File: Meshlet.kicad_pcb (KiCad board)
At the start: 2 copper layers, 60.2 x 39 mm, 114 parts, among them J1 Ext. Notif. Header, J10 STEMMA QT I2C, J11 GPIO Exp., J12 I2C PINHEADER, J13 Ext. Power Header, J2 USB_C_Receptacle_USB2.0_16P, J3 Ext. Power Header, J4 Batt. Header (JST-PH 2.0), J5 SWD, J6 Batt. Header (Picoblade 1.25), J7 GPS Header, J8 User Btn Header, J9 Power Switch, Q1 AO3400A, SW1 BOOTSEL, SW3 RST, U1 W25Q32JVZP, U10 XC6206PxxxMR, U11 XC6206PxxxMR, U2 XC6206PxxxMR, U3 RP2350_60QFN, U4 INA3221, U5 BME280, U6 Wio-SX1262, U7 USBLC6-2SC6, U8 BQ24074RGT, Y1 12.000MHz

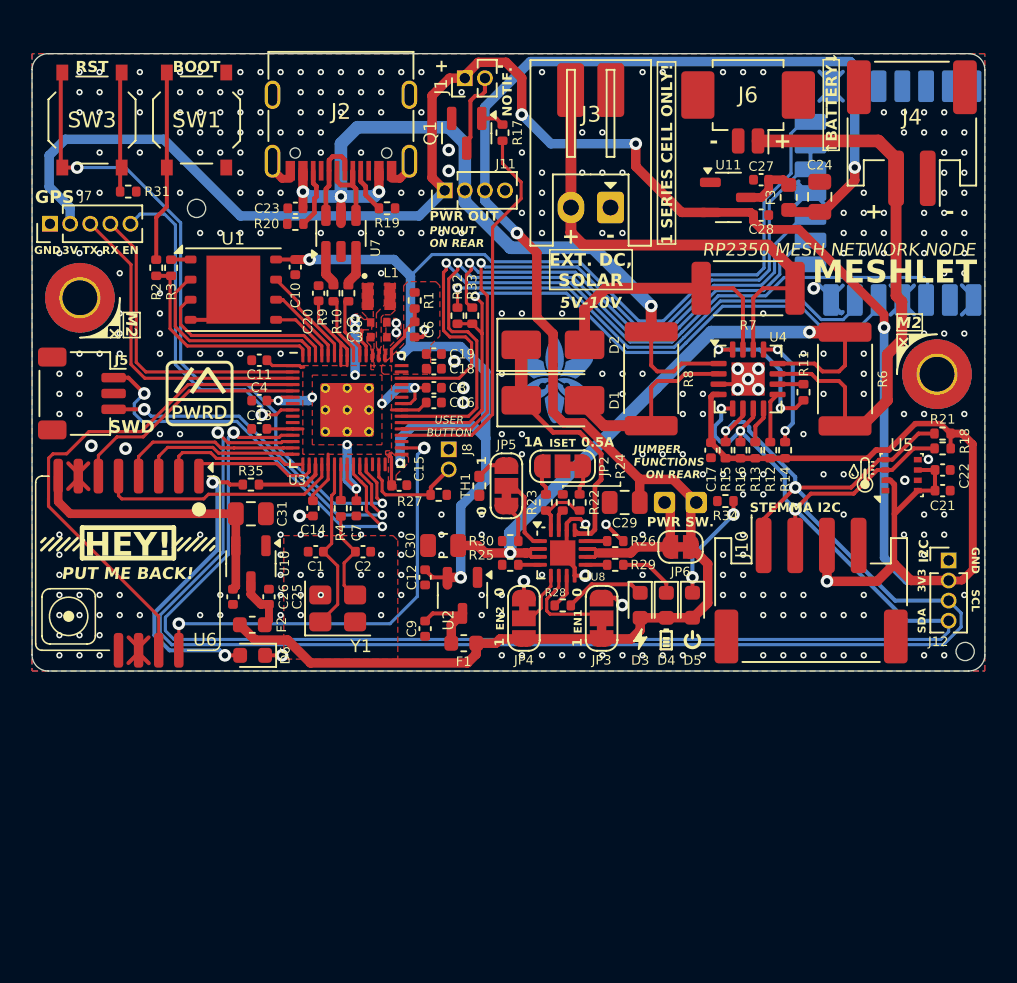
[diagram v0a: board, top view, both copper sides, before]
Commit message: Redesign!
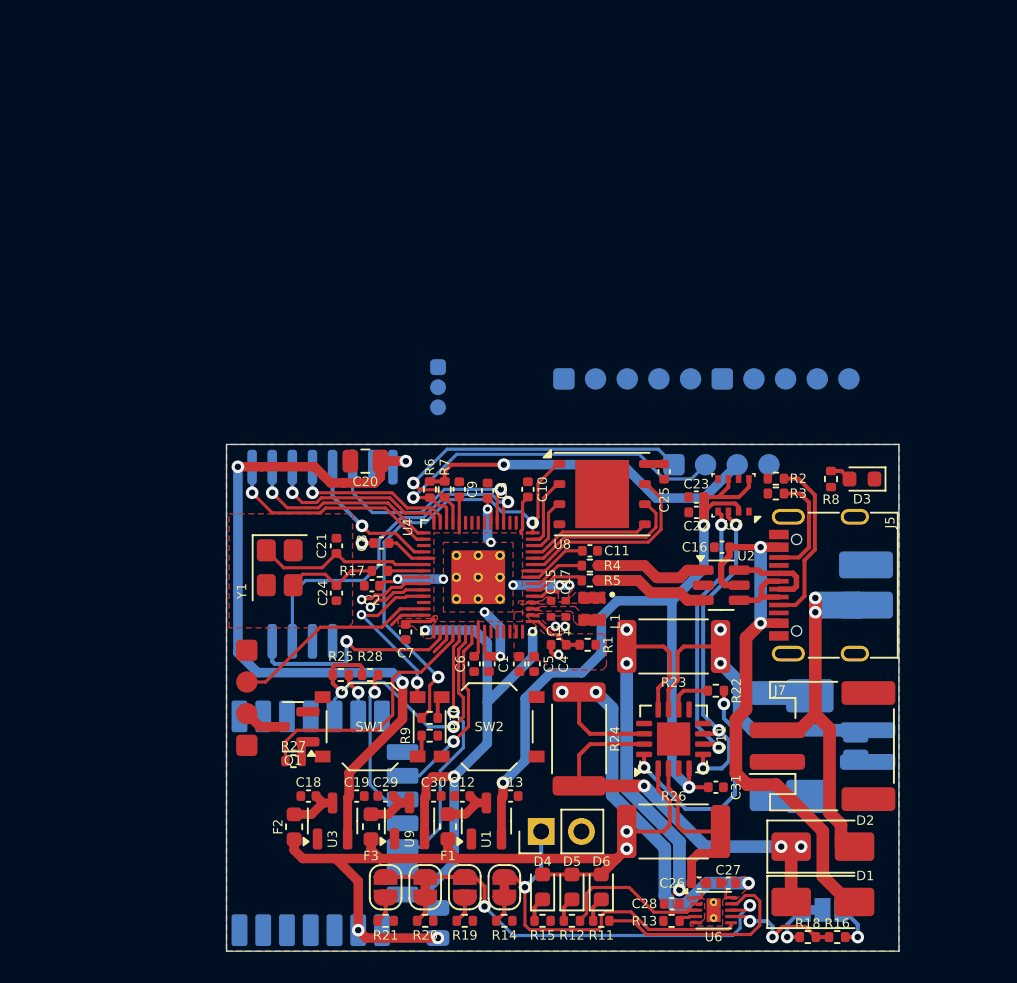
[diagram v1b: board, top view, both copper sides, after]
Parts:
- removed G***: LOGO, Graphics:HalftoneOverlay
- removed J10: STEMMA QT I2C, Connector_JST:JST_PH_S4B-PH-SM4-TB_1x04-1MP_P2.00mm_Horizontal
- removed J8: User Btn Header, Connector_PinHeader_1.27mm:PinHeader_1x02_P1.27mm_Vertical
- removed JP6: PwrSw Bypass, Jumper:SolderJumper-2_P1.3mm_Bridged_RoundedPad1.0x1.5mm
- removed R29, R30, R33, R34, R35: 10k, Resistor_SMD:R_0402_1005Metric
- removed R31: 1k, Resistor_SMD:R_0402_1005Metric
- removed R32: 470R, Resistor_SMD:R_0402_1005Metric
- removed REF** (x2): MountingHole_2.2mm_M2_Pad_TopBottom, MountingHole:MountingHole_2.2mm_M2_Pad_TopBottom
- removed REF** (x2): ToolingHole_1.152mm, MountingHole:ToolingHole_1.152mm
- removed SW3: RST, Button_Switch_SMD:SW_Push_1P1T_XKB_TS-1187A
- removed TH1: Thermistor_NTC, Resistor_SMD:R_0402_1005Metric_Pad0.72x0.64mm_HandSolder
- added C32: 47uF, Capacitor_SMD:C_0805_2012Metric, B.Cu at (135.9, 109.1)
- added J14: Ext. Notif. Header, Connector_PinHeader_2.00mm:PinHeader_1x02_P2.00mm_Vertical, F.Cu at (123.8, 97.9)
- added JP1: TS, Jumper:SolderJumper-2_P1.3mm_Bridged_RoundedPad1.0x1.5mm, F.Cu at (140.1, 106.8)
- added R5: 27R, Resistor_SMD:R_0402_1005Metric, F.Cu at (145.5, 87.5)
- added SW2: BOOTSEL, Button_Switch_SMD:SW_Push_1P1T_XKB_TS-1187A, F.Cu at (139.1, 96.7)
- C1: value 15pF -> 100nF
- C13, C18, C19: value 100nF -> 1uF
- C14: value 100nF -> 4.7uF
- C15, C17: value 100nF -> 4.7uF; footprint Capacitor_SMD:C_0402_1005Metric -> RP2350 Components:C_0402_1005Metric_small_pads
- C2: value 15pF -> 4.7uF
- C20: value 100nF -> 47uF; footprint Capacitor_SMD:C_0402_1005Metric -> Capacitor_SMD:C_0805_2012Metric
- C21: value 100nF -> 15pF
- C24: value 47uF -> 15pF; footprint Capacitor_SMD:C_0805_2012Metric -> Capacitor_SMD:C_0402_1005Metric
- C25, C9: value 1uF -> 100nF
- C26, C27, C28: value 1uF -> 22uF
- C29, C30: value 47uF -> 1uF; footprint Capacitor_SMD:C_0805_2012Metric -> Capacitor_SMD:C_0402_1005Metric
- C3, C5: value 4.7uF -> 100nF; footprint RP2350 Components:C_0402_1005Metric_small_pads -> Capacitor_SMD:C_0402_1005Metric
- C31: value 47uF -> 100nF; footprint Capacitor_SMD:C_0805_2012Metric -> Capacitor_SMD:C_0402_1005Metric
- C6, C7: value 4.7uF -> 100nF
- D3: value PG -> HB
- D4: value CHG -> PV
- D5: value PWR -> CHG
- D6: value HB -> FLT
- J1: value Ext. Notif. Header -> SWD; footprint Connector_PinHeader_1.27mm:PinHeader_1x02_P1.27mm_Vertical -> Connector_PinHeader_1.27mm:PinHeader_1x03_P1.27mm_Vertical; moved to B.Cu
- J11: footprint Connector_PinHeader_1.27mm:PinHeader_1x04_P1.27mm_Vertical -> Connector_PinHeader_2.00mm:PinHeader_1x05_P2.00mm_Vertical; moved to B.Cu
- J12: value I2C PINHEADER -> GPS Header; footprint Connector_PinHeader_1.27mm:PinHeader_1x04_P1.27mm_Vertical -> Connector_PinHeader_2.00mm:PinHeader_1x05_P2.00mm_Vertical; moved to B.Cu
- J13: value Ext. Power Header -> Thermistor Pins
- J2: value USB_C_Receptacle_USB2.0_16P -> User Btn Header; footprint Connector_USB:USB_C_Receptacle_G-Switch_GT-USB-7010ASV -> Connector_PinHeader_2.00mm:PinHeader_1x02_P2.00mm_Vertical
- J3: value Ext. Power Header -> Batt. Header (Picoblade 1.25); footprint Connector_JST:JST_XH_S2B-XH-A_1x02_P2.50mm_Horizontal -> Connector_Molex:Molex_PicoBlade_53261-0271_1x02-1MP_P1.25mm_Horizontal; moved to B.Cu
- J4: moved to B.Cu
- J5: value SWD -> USB_C_Receptacle_USB2.0_16P; footprint Connector_JST:JST_SH_SM03B-SRSS-TB_1x03-1MP_P1.00mm_Horizontal -> Connector_USB:USB_C_Receptacle_G-Switch_GT-USB-7010ASV
- J6: value Batt. Header (Picoblade 1.25) -> STEMMA QT I2C; footprint Connector_Molex:Molex_PicoBlade_53261-0271_1x02-1MP_P1.25mm_Horizontal -> Connector_PinHeader_2.00mm:PinHeader_1x04_P2.00mm_Vertical; moved to B.Cu
- J7: value GPS Header -> Ext. Power Header; footprint Connector_PinHeader_1.27mm:PinHeader_1x05_P1.27mm_Vertical -> Connector_JST:JST_PH_S2B-PH-SM4-TB_1x02-1MP_P2.00mm_Horizontal
- J9: value Power Switch -> Ext. Power Header; footprint Connector_PinHeader_2.00mm:PinHeader_1x02_P2.00mm_Vertical -> Connector_PinHeader_2.54mm:PinHeader_1x02_P2.54mm_Vertical; moved to B.Cu
- JP2: value ISET -> Chemistry Select; moved to B.Cu
- JP3: value EN1 -> SolderJumper_2_Open; footprint Jumper:SolderJumper-3_P1.3mm_Bridged12_RoundedPad1.0x1.5mm -> Jumper:SolderJumper-2_P1.3mm_Open_RoundedPad1.0x1.5mm
- JP4: value EN2 -> SolderJumper_2_Bridged; footprint Jumper:SolderJumper-3_P1.3mm_Bridged12_RoundedPad1.0x1.5mm -> Jumper:SolderJumper-2_P1.3mm_Bridged_RoundedPad1.0x1.5mm
- JP5: value Jumper_3_Bridged12 -> SolderJumper_2_Open; footprint Jumper:SolderJumper-3_P1.3mm_Bridged12_RoundedPad1.0x1.5mm -> Jumper:SolderJumper-2_P1.3mm_Open_RoundedPad1.0x1.5mm
- R10, R9: value 27R -> 1k
- R16: value 10k -> 13k
- R17: value 10k -> 1k
- R18: value 4.7k -> 5.1k
- R19: value 5.1k -> 300
- R2: value 1k -> 5.1k
- R20: value 5.1k -> 600
- R21: value 4.7k -> 1.2k
- R23, R26: value 1k -> PA2512FKF7W0R01E; footprint Resistor_SMD:R_0402_1005Metric -> Resistor_SMD:R_2512_6332Metric
- R24: value 10k -> PA2512FKF7W0R01E; footprint Resistor_SMD:R_0402_1005Metric -> Resistor_SMD:R_2512_6332Metric
- R25: value 10k -> 470R
- R27: value 1k -> 10k
- R3: value 0 -> 5.1k
- R4: value 1k -> 27R
- R6, R7, R8: value PA2512FKF7W0R01E -> 10k; footprint Resistor_SMD:R_2512_6332Metric -> Resistor_SMD:R_0402_1005Metric
- SW1: value BOOTSEL -> RST
- U1: value W25Q32JVZP -> XC6206PxxxMR; footprint Package_SON:WSON-8-1EP_6x5mm_P1.27mm_EP3.4x4.3mm -> Package_TO_SOT_SMD:SOT-23-3
- U10: value XC6206PxxxMR -> ~; footprint Package_TO_SOT_SMD:SOT-23-3 -> RM2:Radio Module 2; moved to B.Cu
- U11: value XC6206PxxxMR -> INA3221; footprint Package_TO_SOT_SMD:SOT-23-3 -> Package_DFN_QFN:Texas_RGV0016A_VQFN-16-1EP_4x4mm_P0.65mm_EP2.1x2.1mm
- U2: value XC6206PxxxMR -> USBLC6-2SC6; footprint Package_TO_SOT_SMD:SOT-23-3 -> Package_TO_SOT_SMD:SOT-23-6
- U3: value RP2350_60QFN -> XC6206PxxxMR; footprint RP2350_60QFN_minimal:RP2350-QFN-60-1EP_7x7_P0.4mm_EP3.4x3.4mm_ThermalVias -> Package_TO_SOT_SMD:SOT-23-3
- U4: value INA3221 -> RP2350_60QFN; footprint Package_DFN_QFN:Texas_RGV0016A_VQFN-16-1EP_4x4mm_P0.65mm_EP2.1x2.1mm -> RP2350_60QFN_minimal:RP2350-QFN-60-1EP_7x7_P0.4mm_EP3.4x3.4mm_ThermalVias
- U5: value BME280 -> Wio-SX1262; footprint Package_LGA:Bosch_LGA-8_2.5x2.5mm_P0.65mm_ClockwisePinNumbering -> Wio-SX1262:Wio-SX1262; moved to B.Cu
- U6: value Wio-SX1262 -> BQ25185; footprint Wio-SX1262:Wio-SX1262 -> Package_DFN_QFN:Texas_DLH0010A_WSON-10-1EP_2.2x2mm_P0.4mm_EP0.9x1.5mm_ThermalVias
- U7: value USBLC6-2SC6 -> BME280; footprint Package_TO_SOT_SMD:SOT-23-6 -> Package_LGA:Bosch_LGA-8_2.5x2.5mm_P0.65mm_ClockwisePinNumbering
- U8: value BQ24074RGT -> W25Q32JVZP; footprint Package_DFN_QFN:VQFN-16-1EP_3x3mm_P0.5mm_EP1.6x1.6mm -> Package_SON:WSON-8-1EP_6x5mm_P1.27mm_EP3.4x4.3mm
- U9: value ~ -> XC6206PxxxMR; footprint RM2:Radio Module 2 -> Package_TO_SOT_SMD:SOT-23-3; moved to F.Cu
- moved J7 58.9 mm to (160.2, 97.9)
- moved U9 57.4 mm to (134.1, 102.6)
- moved J5 49.3 mm to (161.2, 87.7), turned to 90 degrees
- moved F3 47.7 mm to (131.7, 103.0)
- moved J13 47.0 mm to (142.4, 103.3), turned to 90 degrees
- moved R21 46.7 mm to (132.6, 108.9), turned to 180 degrees
- moved R19 45.3 mm to (137.6, 108.9), turned to 180 degrees
- moved R20 44.8 mm to (135.1, 108.9), turned to 180 degrees
- moved C27 44.5 mm to (154.2, 106.6)
- moved C28 43.9 mm to (150.7, 107.9), turned to 180 degrees
- moved U6 43.0 mm to (153.3, 108.3), turned to 0 degrees
- moved U5 42.3 mm to (122.8, 80.3), turned to 0 degrees
- moved R2 41.3 mm to (157.2, 81.0), turned to 180 degrees
- moved R3 40.8 mm to (157.2, 82.0), turned to 0 degrees
- moved SW1 39.9 mm to (131.6, 96.7), turned to 0 degrees
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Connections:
- C1 pad 1: GND -> +1V1
- C1 pad 2: XIN -> GND
- C12 pad 1: /Pi +3V3 -> Net-(U1-VI)
- C13 pad 1: /Pi +3V3 -> +3V3
- C14 pad 1: /Pi +3V3 -> Net-(U4-VREG_AVDD)
- C16 pad 1: /Pi +3V3 -> USB_RAW
- C17 pad 1: GND -> +1V1
- C17 pad 2: +3V3 -> GND
- C18 pad 1: /Pi +3V3 -> Net-(U3-VI)
- C19 pad 1: /Pi +3V3 -> /LoRa +3V3
- C2 pad 1: GND -> +1V1
- C2 pad 2: Net-(C2-Pad2) -> GND
- C20 pad 1: /Pi +3V3 -> GND
- C20 pad 2: GND -> /LoRa +3V3
- C21 pad 1: +3V3 -> GND
- C21 pad 2: GND -> XIN
- C23 pad 1: INA_IN3- -> +3V3
- C24 pad 2: BMS_OUT -> Net-(C24-Pad2)
- C25 pad 1: Net-(U10-VI) -> /Pi +3V3
- C26 pad 1: /LoRa +3V3 -> BMS_INA
- C27 pad 1: Net-(U11-VI) -> VBUS_OUT
- C28 pad 1: +3V3 -> BATT
- C29 pad 1: BMS_OUT -> Net-(U9-VI)
- C3 pad 1: /Pi +3V3 -> +1V1
- C30 pad 1: INA_IN1+ -> /Pi +3V3
- C31 pad 2: /LoRa +3V3 -> +3V3
- C4 pad 1: +1V1 -> /Pi +3V3
- C5 pad 1: +1V1 -> /Pi +3V3
- C6 pad 1: Net-(U3-VREG_AVDD) -> /Pi +3V3
- C7 pad 1: +1V1 -> /Pi +3V3
- C8 pad 1: +1V1 -> /Pi +3V3
- C9 pad 1: Net-(U2-VI) -> /Pi +3V3
- D1 pad 1: VBUS -> VBUS_INA
- D1 pad 2: INA_IN3+ -> USB_RAW
- D2 pad 1: VBUS -> VBUS_INA
- D2 pad 2: INA_IN2+ -> Net-(D2-A)
- D3 pad 1: Net-(D3-K) -> GND
- D3 pad 2: BMS_OUT -> Net-(D3-A)
- D6 pad 1: GND -> Net-(D6-K)
- D6 pad 2: Net-(D6-A) -> BMS_OUT
- F1 pad 2: Net-(U2-VI) -> Net-(U1-VI)
- F2 pad 2: Net-(U10-VI) -> Net-(U3-VI)
- F3 pad 2: Net-(U11-VI) -> Net-(U9-VI)
- J1 pad 1: +3V3 -> SWCLK
- J1 pad 2: Net-(J1-Pin_2) -> GND
- J11 pad 1: +3V3 -> GP4
- J11 pad 2: INA_IN3- -> GP16
- J11 pad 3: BMS_OUT -> GP18
- J11 pad 4: GND -> GP19
- J12 pad 3: I2C_SCL -> GPS_TX
- J12 pad 4: I2C_SDA -> GPS_RX
- J13 pad 1: GND -> THERM
- J13 pad 2: INA_IN2- -> GND
- J3 pad 2: INA_IN2- -> BATT_INA
- J4 pad 2: INA_IN1- -> BATT_INA
- J6 pad 1: INA_IN1- -> I2C_SDA
- J6 pad 2: GND -> I2C_SCL
- J7 pad 2: +3V3 -> Net-(D2-A)
- J9 pad 1: Net-(J9-Pin_1) -> GND
- J9 pad 2: BMS_OUT -> Net-(D2-A)
- JP3 pad 1: BMS_OUT -> Net-(JP3-A)
- JP3 pad 2: BMS_EN1 -> ISET
- JP4 pad 1: GND -> Net-(JP4-A)
- JP4 pad 2: BMS_EN2 -> ISET
- JP5 pad 2: Net-(JP5-C) -> ISET
- L1 pad 2: Net-(U3-VREG_LX) -> Net-(U4-VREG_LX)
- Q1 pad 3: Net-(J1-Pin_2) -> Net-(J14-Pin_2)
- R1 pad 2: Net-(U3-VREG_AVDD) -> Net-(U4-VREG_AVDD)
- R10 pad 1: USB_DN -> Net-(R10-Pad1)
- R10 pad 2: Net-(U3-USB_DM) -> QSPI_SS
- R11 pad 1: INA_VPU -> Net-(U6-STAT1)
- R11 pad 2: INA_PV -> Net-(D6-K)
- R12 pad 1: +3V3 -> Net-(U6-STAT2)
- R12 pad 2: INA_CRIT -> Net-(D5-K)
- R13 pad 1: +3V3 -> GND
- R13 pad 2: INA_WARN -> Net-(U6-CE)
- R14 pad 1: +3V3 -> Net-(JP1-B)
- R14 pad 2: INA_TC -> GND
- R15 pad 1: +3V3 -> Net-(D4-K)
- R15 pad 2: I2C_SCL -> GND
- R16 pad 1: +3V3 -> VSET
- R16 pad 2: I2C_SDA -> Net-(JP2-B)
- R17 pad 1: NOTIFY -> Net-(C24-Pad2)
- R17 pad 2: Net-(Q1-G) -> XOUT
- R18 pad 1: I2C_SDA -> Net-(JP2-A)
- R18 pad 2: +3V3 -> VSET
- R19 pad 1: Net-(J2-CC1) -> GND
- R19 pad 2: GND -> Net-(JP3-A)
- R2 pad 1: Net-(R2-Pad1) -> Net-(J5-CC1)
- R2 pad 2: QSPI_SS -> GND
- R20 pad 2: Net-(J2-CC2) -> Net-(JP4-A)
- R21 pad 1: I2C_SCL -> GND
- R21 pad 2: +3V3 -> Net-(JP5-A)
- R22 pad 1: Net-(U8-ISET) -> INA_VPU
- R22 pad 2: Net-(JP2-A) -> INA_PV
- R23 pad 1: Net-(U8-ISET) -> BATT
- R23 pad 2: Net-(JP2-B) -> BATT_INA
- R24 pad 1: GND -> VBUS_INA
- R24 pad 2: Net-(U8-ITERM) -> VBUS_OUT
- R25 pad 1: Net-(U8-~{CE}) -> GP24
- R25 pad 2: GND -> Net-(U10-DO)
- R26 pad 1: GND -> BMS_INA
- R26 pad 2: Net-(U8-ILIM) -> BMS_OUT
- R27 pad 1: USER_BTN -> NOTIFY
- R27 pad 2: GND -> Net-(Q1-G)
- R28 pad 1: Net-(U8-~{PGOOD}) -> GP24
- R28 pad 2: Net-(D3-K) -> Net-(U10-IRQ)
- R3 pad 1: Net-(U1-~{CS}) -> GND
- R3 pad 2: QSPI_SS -> Net-(J5-CC2)
- R4 pad 1: Net-(C2-Pad2) -> USB_DP
- R4 pad 2: XOUT -> Net-(U4-USB_DP)
- R6 pad 1: INA_IN1+ -> +3V3
- R6 pad 2: INA_IN1- -> I2C_SCL
- R7 pad 1: INA_IN2+ -> +3V3
- R7 pad 2: INA_IN2- -> I2C_SDA
- R8 pad 1: INA_IN3+ -> Net-(D3-A)
- R8 pad 2: INA_IN3- -> Net-(U4-GPIO14)
- R9 pad 1: USB_DP -> Net-(R9-Pad1)
- R9 pad 2: Net-(U3-USB_DP) -> GND
- SW1 pad 1: Net-(R2-Pad1) -> Net-(U4-RUN)
- SW1 pad 2: GND -> Net-(R9-Pad1)
- U1 pad 1: Net-(U1-~{CS}) -> GND
- U1 pad 2: QSPI_SD1 -> +3V3
- U1 pad 3: QSPI_SD2 -> Net-(U1-VI)
- U10 pad 2: /LoRa +3V3 -> unconnected-(U10-NC-Pad2)
- U10 pad 3: Net-(U10-VI) -> GP29
- U11 pad 1: GND -> BMS_OUT
- U11 pad 2: +3V3 -> BMS_INA
- U11 pad 3: Net-(U11-VI) -> GND
- U2 pad 1: GND -> USB_DP
- U2 pad 2: /Pi +3V3 -> GND
- U2 pad 3: Net-(U2-VI) -> USB_DN
- U3 pad 1: /Pi +3V3 -> GND
- U3 pad 2: GPS_RX -> /LoRa +3V3
- U3 pad 3: GPS_TX -> Net-(U3-VI)
- U4 pad 1: INA_IN3- -> /Pi +3V3
- U4 pad 10: INA_PV -> unconnected-(U4-GPIO7-Pad10)
- U4 pad 11: INA_IN1- -> /Pi +3V3
- U4 pad 12: INA_IN1+ -> I2C_SDA
- U4 pad 13: INA_TC -> I2C_SCL
- U4 pad 14: INA_IN2- -> LORA_SCK
- U4 pad 15: INA_IN2+ -> LORA_MOSI
- U4 pad 16: INA_VPU -> LORA_MISO
- U4 pad 17: GND -> LORA_RF_SW
- U4 pad 2: INA_IN3+ -> GPS_RX
- U4 pad 3: GND -> GPS_TX
- U4 pad 4: +3V3 -> LORA_BUSY
- U4 pad 5: I2C_SDA -> LORA_CS
- U4 pad 6: I2C_SCL -> +1V1
- U4 pad 7: I2C_SDA -> GPS_EN
- U4 pad 8: INA_WARN -> GP4
- U4 pad 9: INA_CRIT -> unconnected-(U4-GPIO6-Pad9)
- U5 pad 1: GND -> LORA_RF_SW
- U5 pad 2: +3V3 -> LORA_MISO
- U5 pad 3: I2C_SDA -> LORA_MOSI
- U5 pad 4: I2C_SCL -> LORA_SCK
- U5 pad 5: GND -> LORA_RST
- U5 pad 6: +3V3 -> LORA_CS
- U5 pad 8: +3V3 -> /LoRa +3V3
- U6 pad 1: LORA_RF_SW -> BMS_INA
- U6 pad 10: GND -> VBUS_OUT
- U6 pad 11: LORA_BUSY -> GND
- U6 pad 2: LORA_MISO -> BATT
- U6 pad 3: LORA_MOSI -> Net-(U6-STAT2)
- U6 pad 4: LORA_SCK -> Net-(U6-CE)
- U6 pad 5: LORA_RST -> GND
- U6 pad 6: LORA_CS -> THERM
- U6 pad 7: GND -> VSET
- U6 pad 8: /LoRa +3V3 -> ISET
- U6 pad 9: unconnected-(U6-ANT-Pad9) -> Net-(U6-STAT1)
- U7 pad 1: USB_DP -> GND
- U7 pad 2: GND -> +3V3
- U7 pad 3: USB_DN -> I2C_SDA
- U7 pad 4: USB D- -> I2C_SCL
- U7 pad 5: INA_IN3- -> GND
- U7 pad 6: USB D+ -> +3V3
- U8 pad 1: Net-(JP5-C) -> QSPI_SS
- U8 pad 2: INA_IN1+ -> QSPI_SD1
- U8 pad 3: INA_IN1+ -> QSPI_SD2
- U8 pad 4: Net-(U8-~{CE}) -> GND
- U8 pad 5: BMS_EN2 -> QSPI_SD0
- U8 pad 6: BMS_EN1 -> QSPI_SCLK
- U8 pad 7: Net-(U8-~{PGOOD}) -> QSPI_SD3
- U8 pad 8: GND -> /Pi +3V3
- U8 pad 9: Net-(U8-~{CHG}) -> GND
- U9 pad 2: unconnected-(U9-NC-Pad2) -> /Pi +3V3
- U9 pad 3: GP29 -> Net-(U9-VI)
- Y1 pad 3: Net-(C2-Pad2) -> Net-(C24-Pad2)
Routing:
- net +3V3: track 155.0 -> 76.2 mm
- net I2C_SCL: track 110.2 -> 41.2 mm
- net I2C_SDA: track 109.1 -> 43.3 mm
- net BMS_OUT: track 110.8 -> 51.2 mm, vias 2 -> 4
- net INA_IN3-: track 48.5 -> 0.00 mm, vias 4 -> 0
- net GP29: track 48.1 -> 0.00 mm, vias 1 -> 0
- net GND: track 49.4 -> 1.75 mm, vias 323 -> 4
- net /Pi +3V3: track 99.3 -> 53.8 mm, vias 4 -> 3
- net Net-(U3-RUN): track 44.2 -> 0.00 mm, vias 2 -> 0
- net INA_IN1+: track 40.8 -> 0.00 mm, vias 2 -> 0
- net INA_IN1-: track 35.4 -> 0.00 mm
- net USB_RAW: track 0.00 -> 34.9 mm, vias 0 -> 2
- net INA_IN2-: track 31.4 -> 0.00 mm
- net GP25: track 42.9 -> 11.8 mm
- net Net-(D2-A): track 0.00 -> 30.9 mm, vias 0 -> 2
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- added copper zone on F.Cu, net BATT
- added copper zone on F.Cu, net BMS_INA
- added copper zone on In1.Cu, net GND
- added copper zone on In2.Cu, net GND
- added copper zone on F.Cu, net Net-(U4-VREG_LX)
- added copper zone on F.Cu, net VBUS_OUT
- removed copper zone on F.Cu, net Net-(U3-VREG_LX)
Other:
- board size 60.2 x 39 mm -> 42.5 x 32 mm
- copper layers 2 -> 4
- board text removed: "!"
- board text removed: "*4V4 MAX"
- board text removed: "*BMS"
- board text removed: "+"
- board text removed: "-"
- board text removed: "0"
- board text removed: "0.5A"
- board text removed: "1"
- board text removed: "1 SERIES CELL ONLY!"
- board text removed: "1A"
- board text removed: "3V"
- board text removed: "3V3"
- board text removed: "5V-10V"
- board text removed: ":"
- board text removed: "BOOT"
- board text removed: "Charge Rate (default 0.5A, 1A jumped)"
- board text removed: "DESIGNED IN"
- board text removed: "EDMONTON, AB"
- board text removed: "EN"
- board text removed: "EN1"
- board text removed: "EN1 (see datasheet, default high)"
- board text removed: "EN2"
- board text removed: "EN2 (see datasheet, default low)"
- board text removed: "EP V0.2"
- board text removed: "EXT. DC, SOLAR"
- board text removed: "EXTERNAL NOTIFS"
- board text removed: "GND"
- board text removed: "GP0"
- board text removed: "GP1"
- board text removed: "GP22"
- board text removed: "GP5"
- board text removed: "GPS"
- board text removed: "HEY!"
- board text removed: "I HOPE YOU HAVE A LONG ENOUGH USB CABLE"
- board text removed: "I2C"
- board text removed: "ISET"
- board text removed: "JP1:"
- board text removed: "JP2:"
- board text removed: "JP3:"
- board text removed: "JP4:"
- board text removed: "JP5:"
- board text removed: "JUMPER FUNCTIONS"
- board text removed: "LITHIUM ION & POLYMER"
- board text removed: "M2"
- board text removed: "MESH NETWORK NODE RP2350 MESH NETWORK NODE RP2350"
- board text removed: "MESHLET"
- board text removed: "MULTIPLE CELLS IN PARALLEL ARE OK IF YOU KNOW WHAT YOU'RE DOING"
- board text removed: "NOTIF."
- board text removed: "ON REAR"
- board text removed: "OUTPUTS ONLY! **"
- board text removed: "PINOUT ON REAR"
- board text removed: "PUT ME BACK!"
- board text removed: "PWR OUT"
- board text removed: "PWR SW."
- board text removed: "Pwr Sw. Bypass (cut to add pwr switch)"
- board text removed: "RP2350 MESH NETWORK NODE"
- board text removed: "RPI RM2"
- board text removed: "RST"
- board text removed: "RX"
- board text removed: "SCL"
- board text removed: "SDA"
- board text removed: "STEMMA I2C"
- board text removed: "SWD"
- board text removed: "THE BQ24074 IS A 1-CELL SERIES CHARGER ONLY!"
- board text removed: "TX"
- board text removed: "Thermistor (cut & jump to 1 if present)"
- board text removed: "USB"
- board text removed: "USER BUTTON"
- board text removed: "VERSION 0.2"
- board text removed: "https://5panel.dance/Meshlet"
- board text removed: "×"
- board text removed: "×1"
- board text removed: "↑BATTERY↓"

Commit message: 4 layer ver. complete!
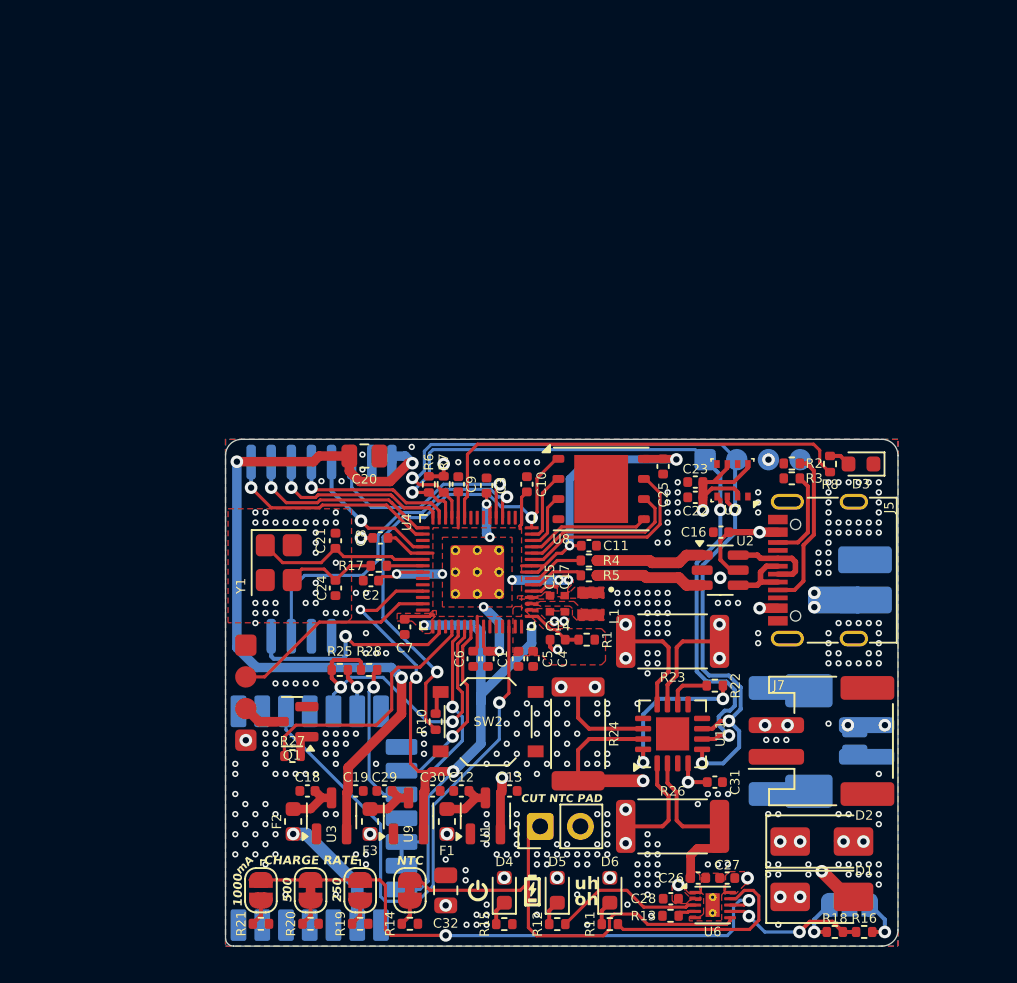
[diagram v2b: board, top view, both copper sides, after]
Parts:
- removed J1: SWD, Connector_PinHeader_1.27mm:PinHeader_1x03_P1.27mm_Vertical
- removed J11: GPIO Exp., Connector_PinHeader_2.00mm:PinHeader_1x05_P2.00mm_Vertical
- removed J12: GPS Header, Connector_PinHeader_2.00mm:PinHeader_1x05_P2.00mm_Vertical
- removed R9: 1k, Resistor_SMD:R_0402_1005Metric
- removed SW1: RST, Button_Switch_SMD:SW_Push_1P1T_XKB_TS-1187A
- C32: moved to F.Cu
- moved JP5 7.88 mm to (124.7, 107.0)
- moved R21 7.88 mm to (124.7, 109.1)
- moved JP4 7.24 mm to (127.8, 107.0)
- moved R20 7.24 mm to (127.8, 109.1)
- moved JP3 6.61 mm to (131.0, 107.0)
- moved R19 6.61 mm to (131.0, 109.1)
- moved JP1 5.97 mm to (134.1, 107.0)
- moved R14 5.97 mm to (134.1, 109.1)
- moved D4 2.43 mm to (140.1, 107.0)
- moved R15 2.43 mm to (140.1, 109.2)
- moved C32 2.12 mm to (136.4, 107.0)
- moved J6 2.00 mm to (152.8, 79.8)
- moved R18 1.74 mm to (161.0, 109.6)
- moved JP2 1.74 mm to (161.9, 107.9)
- moved R16 1.74 mm to (162.8, 109.6)
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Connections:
- J6 pad 1: I2C_SDA -> I2C_SCL
- J6 pad 2: I2C_SCL -> I2C_SDA
- R6 pad 1: +3V3 -> /Pi +3V3
- R7 pad 1: +3V3 -> /Pi +3V3
- R8 pad 2: Net-(U4-GPIO14) -> HB
- U4 pad 10: unconnected-(U4-GPIO7-Pad10) -> HB
- U4 pad 18: Net-(U4-GPIO14) -> unconnected-(U4-GPIO14-Pad18)
- U4 pad 26: Net-(U4-RUN) -> /Pi +3V3
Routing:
- net /Pi +3V3: track 53.8 -> 102.9 mm, vias 3 -> 8
- net GP29: track 0.00 -> 36.4 mm, vias 0 -> 1
- net HB: track 0.00 -> 28.4 mm
- net I2C_SDA: track 43.3 -> 54.6 mm
- net Net-(U4-RUN): track 11.1 -> 0.00 mm, vias 2 -> 0
- net ISET: track 28.6 -> 37.3 mm
- net I2C_SCL: track 41.2 -> 47.9 mm
- net THERM: track 22.7 -> 29.1 mm, vias 1 -> 0
- net BMS_OUT: track 51.2 -> 45.8 mm, vias 4 -> 9
- net INA_VPU: track 14.9 -> 10.1 mm
- net +3V3: track 76.2 -> 71.7 mm, vias 4 -> 5
- net SWCLK: track 4.35 -> 0.00 mm, vias 1 -> 0
- net SWDIO: track 3.81 -> 0.00 mm, vias 1 -> 0
- net VBUS_OUT: track 29.2 -> 26.7 mm
- net GP18: track 2.30 -> 0.00 mm
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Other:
- outline, holes or cut-outs redrawn
- board text added: "1000"
- board text added: "250"
- board text added: "500"
- board text added: "CHARGE RATE"
- board text added: "CHEM"
- board text added: "CUT NTC PAD"
- board text added: "LiFePO4"
- board text added: "LiPo"
- board text added: "NTC"
- board text added: "mA"
- board text added: "oh"
- board text added: "uh"
